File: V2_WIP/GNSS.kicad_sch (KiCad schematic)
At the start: 12 parts, among them J301 USB_B_Micro, U301 USBLC6-2SC6, U401 NEO-M9N

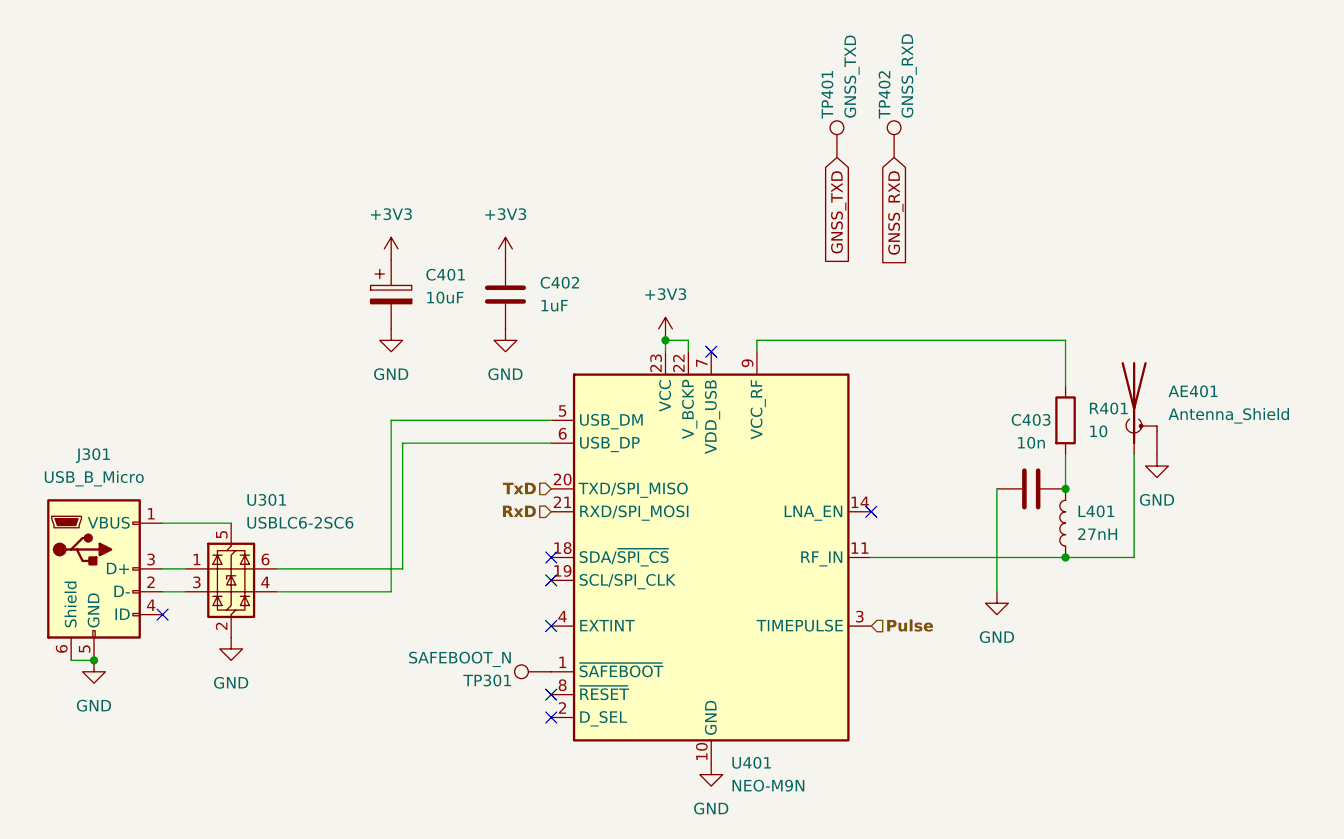
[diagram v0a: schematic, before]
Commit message: minor schematic changes
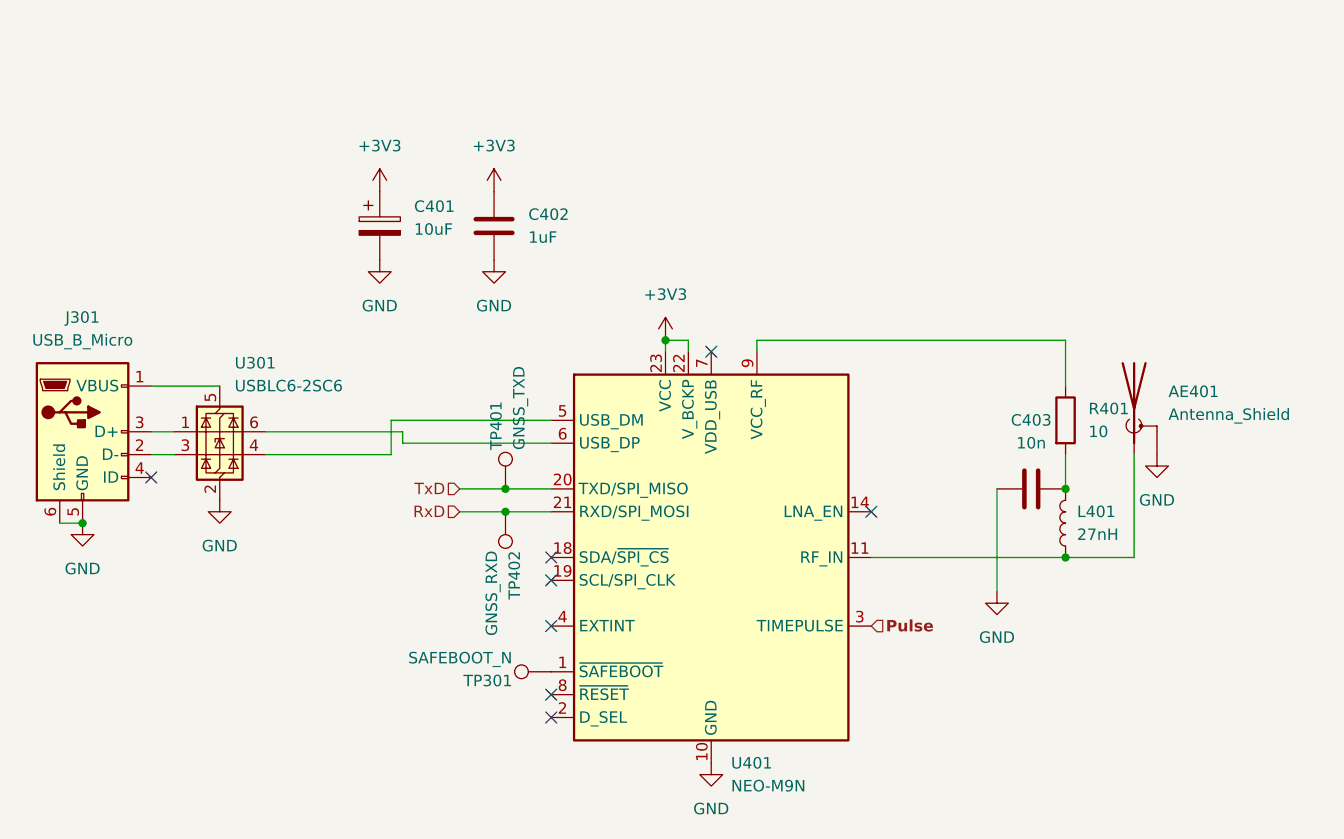
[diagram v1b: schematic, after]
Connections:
- net GNSS_RXD is gone; now on net RxD: TP402.1
- net GNSS_TXD is gone; now on net TxD: TP401.1
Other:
- moved on the sheet: C401, C402, J301, TP401, TP402, U301
